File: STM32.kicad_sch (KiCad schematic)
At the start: 28 parts, among them J1 USB_C_Receptacle_USB2.0_16P, SW1 SW_SPST, SW2 SW_SPST, U2 ADUM4160, U7 USBLC6-2SC6, U8 DS8572-33S5, U9 STM32F072CBTx

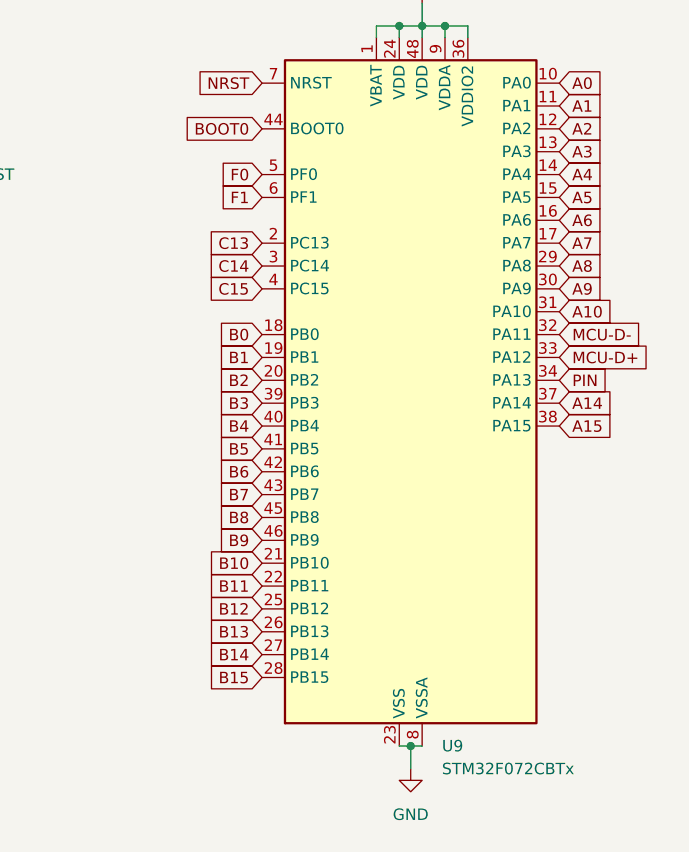
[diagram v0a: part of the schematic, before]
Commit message: draf 1 for sims
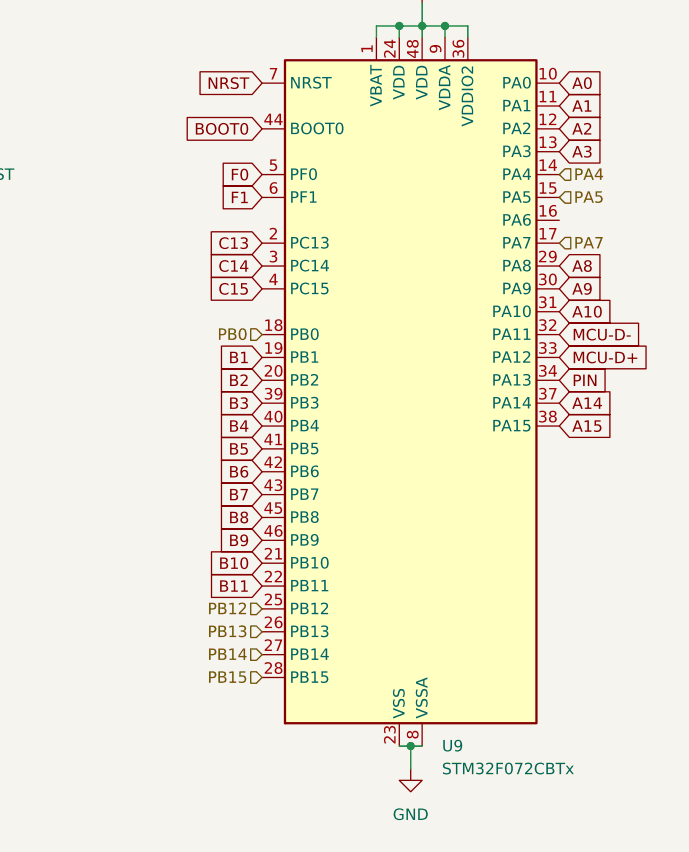
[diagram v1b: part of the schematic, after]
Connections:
- net A4 renamed PA4
- net A5 renamed PA5
- net A6: no longer names the net of U9.16 (PA6)
- net A7 renamed PA7
- net B0 renamed PB0
- net B12 renamed PB12
- net B13 renamed PB13
- net B14 renamed PB14
- net B15 renamed PB15
